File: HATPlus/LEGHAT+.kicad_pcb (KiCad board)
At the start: 4 copper layers, 65 x 56.5 mm, 28 parts, among them J1 Conn_02x20_Odd_Even, J2 Conn_01x02, J3 Conn_01x08, Q2 CSD18540Q5B, SW1 SW_Push, U4 LTC4373IDD-PBF

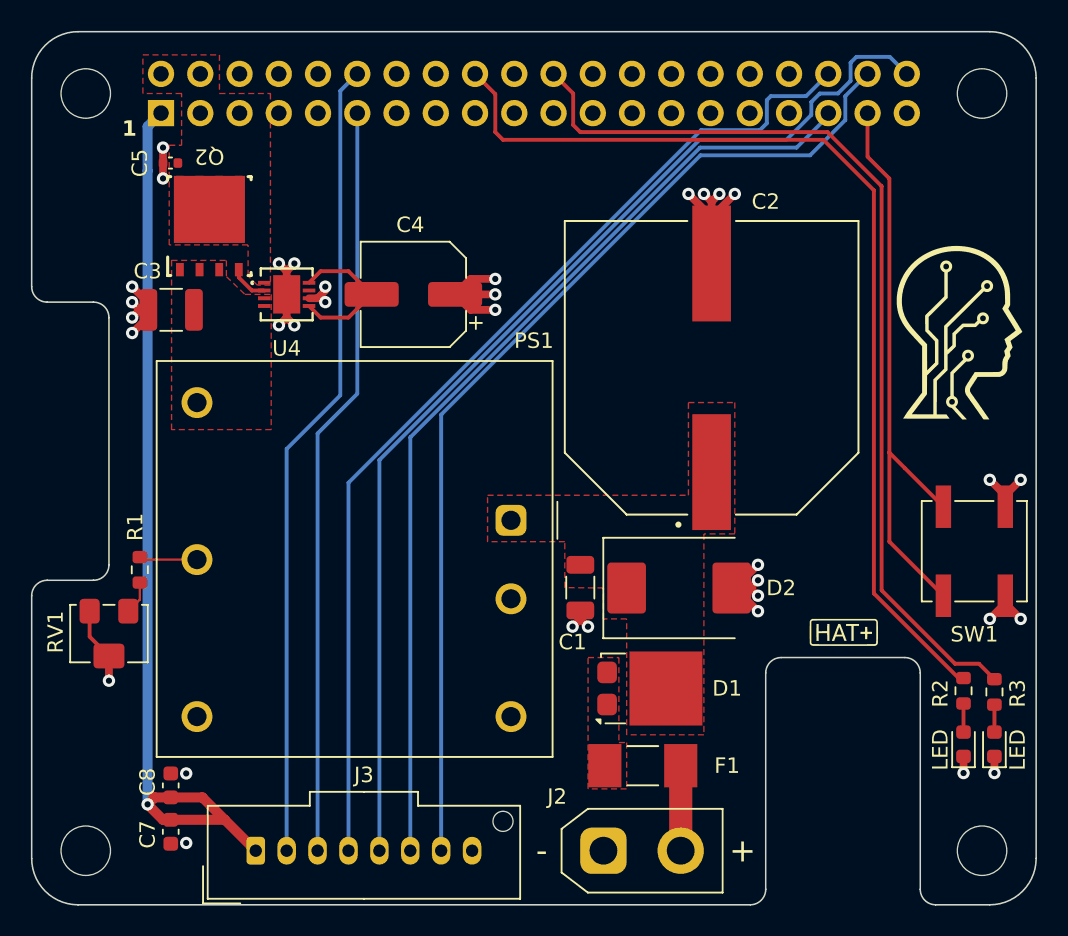
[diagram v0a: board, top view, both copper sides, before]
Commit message: First Draft
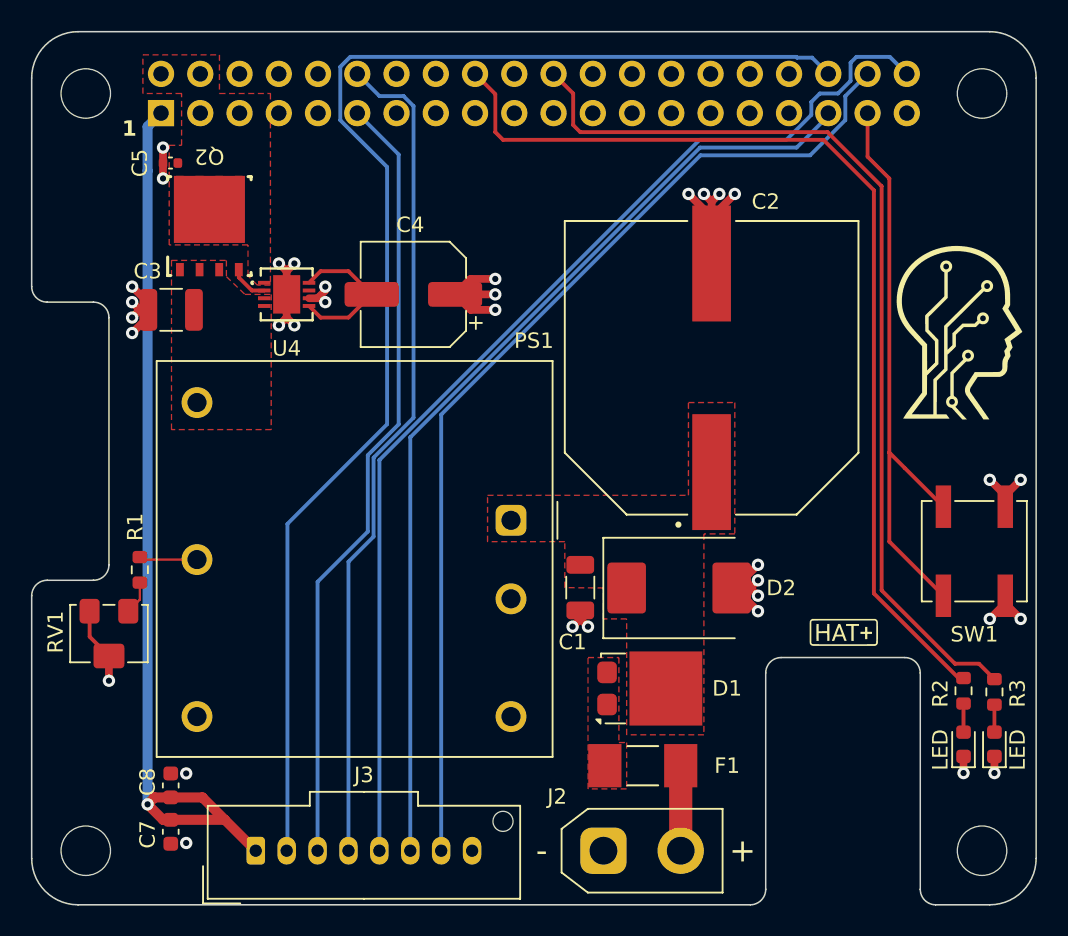
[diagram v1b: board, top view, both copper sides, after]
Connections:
- J1 pad 12: /SPI1_CSn2 -> /SPI1_CSn0
- J1 pad 36: /SPI1_CSn0 -> /SPI1_CSn2
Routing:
- net /SPI1_CSn2: track 52.2 -> 87.0 mm
- net /SPI1_CSn0: track 66.7 -> 54.4 mm
- net /SPI1_CSn1: track 48.8 -> 51.0 mm
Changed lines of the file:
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@@
 			(layers "*.Cu" "*.Mask")
 			(remove_unused_layers no)
-			(net "/SPI1_CSn2")
+			(net "/SPI1_CSn0")
 			(pinfunction "Pin_12_12")
 			(pintype "passive")
@@
 			(layers "*.Cu" "*.Mask")
 			(remove_unused_layers no)
-			(net "/SPI1_CSn0")
+			(net "/SPI1_CSn2")
 			(pinfunction "Pin_36_36")
 			(pintype "passive")
@@
 	)
 	(segment
+		(start 19.97 2.274365)
+		(end 19.97 5.725635)
+		(width 0.25)
+		(layer "B.Cu")
+		(net "/SPI1_CSn2")
+	)
+	(segment
+		(start 51.55 2.73)
+		(end 50.5 1.68)
+		(width 0.25)
+		(layer "B.Cu")
+		(net "/SPI1_CSn2")
+	)
+	(segment
+		(start 49.515635 1.68)
+		(end 49.465635 1.63)
+		(width 0.25)
+		(layer "B.Cu")
+		(net "/SPI1_CSn2")
+	)
+	(segment
+		(start 20.614365 1.63)
+		(end 19.97 2.274365)
+		(width 0.25)
+		(layer "B.Cu")
+		(net "/SPI1_CSn2")
+	)
+	(segment
+		(start 23 8.755635)
+		(end 23 25.4)
+		(width 0.25)
+		(layer "B.Cu")
+		(net "/SPI1_CSn2")
+	)
+	(segment
+		(start 19.97 5.725635)
+		(end 23 8.755635)
+		(width 0.25)
+		(layer "B.Cu")
+		(net "/SPI1_CSn2")
+	)
+	(segment
+		(start 16.55 52.95)
+		(end 16.5 53)
+		(width 0.15)
+		(layer "B.Cu")
+		(net "/SPI1_CSn2")
+	)
+	(segment
+		(start 16.55 31.85)
+		(end 16.55 52.95)
+		(width 0.25)
+		(layer "B.Cu")
+		(net "/SPI1_CSn2")
+	)
+	(segment
+		(start 23 25.4)
+		(end 16.55 31.85)
+		(width 0.25)
+		(layer "B.Cu")
+		(net "/SPI1_CSn2")
+	)
+	(segment
+		(start 50.5 1.68)
+		(end 49.515635 1.68)
+		(width 0.25)
+		(layer "B.Cu")
+		(net "/SPI1_CSn2")
+	)
+	(segment
+		(start 49.465635 1.63)
+		(end 20.614365 1.63)
+		(width 0.25)
+		(layer "B.Cu")
+		(net "/SPI1_CSn2")
+	)
+	(segment
+		(start 23.75 25.40901)
+		(end 21.75 27.40901)
+		(width 0.25)
+		(layer "B.Cu")
+		(net "/SPI1_CSn1")
+	)
+	(segment
+		(start 23.75 7.95)
+		(end 23.75 25.40901)
+		(width 0.25)
+		(layer "B.Cu")
+		(net "/SPI1_CSn1")
+	)
+	(segment
+		(start 18.5 35.6)
+		(end 18.5 53)
+		(width 0.25)
+		(layer "B.Cu")
+		(net "/SPI1_CSn1")
+	)
+	(segment
+		(start 21.07 5.27)
+		(end 23.75 7.95)
+		(width 0.25)
+		(layer "B.Cu")
+		(net "/SPI1_CSn1")
+	)
+	(segment
+		(start 21.75 27.40901)
+		(end 21.75 32.35)
+		(width 0.25)
+		(layer "B.Cu")
+		(net "/SPI1_CSn1")
+	)
+	(segment
+		(start 21.75 32.35)
+		(end 18.5 35.6)
+		(width 0.25)
+		(layer "B.Cu")
+		(net "/SPI1_CSn1")
+	)
+	(segment
+		(start 24.71 4.814365)
+		(end 24.71 24.97934)
+		(width 0.25)
+		(layer "B.Cu")
+		(net "/SPI1_CSn0")
+	)
+	(segment
+		(start 20.5 34.3)
+		(end 20.5 53)
+		(width 0.25)
+		(layer "B.Cu")
+		(net "/SPI1_CSn0")
+	)
+	(segment
+		(start 24.065635 4.17)
+		(end 24.71 4.814365)
+		(width 0.25)
+		(layer "B.Cu")
+		(net "/SPI1_CSn0")
+	)
+	(segment
 		(start 21.07 2.73)
-		(end 19.97 3.83)
-		(width 0.25)
-		(layer "B.Cu")
-		(net "/SPI1_CSn2")
-	)
-	(segment
-		(start 19.97 23.53)
-		(end 16.5 27)
-		(width 0.25)
-		(layer "B.Cu")
-		(net "/SPI1_CSn2")
-	)
-	(segment
-		(start 19.97 3.83)
-		(end 19.97 23.53)
-		(width 0.25)
-		(layer "B.Cu")
-		(net "/SPI1_CSn2")
-	)
-	(segment
-		(start 16.5 27)
-		(end 16.5 53)
-		(width 0.25)
-		(layer "B.Cu")
-		(net "/SPI1_CSn2")
-	)
-	(segment
-		(start 21.07 23.43)
-		(end 18.5 26)
-		(width 0.25)
-		(layer "B.Cu")
-		(net "/SPI1_CSn1")
-	)
-	(segment
-		(start 21.07 5.27)
-		(end 21.07 23.43)
-		(width 0.25)
-		(layer "B.Cu")
-		(net "/SPI1_CSn1")
-	)
-	(segment
-		(start 18.5 26)
-		(end 18.5 53)
-		(width 0.25)
-		(layer "B.Cu")
-		(net "/SPI1_CSn1")
-	)
-	(segment
-		(start 47.83 4.17)
-		(end 47.57 4.43)
+		(end 22.51 4.17)
 		(width 0.25)
 		(layer "B.Cu")
@@
 	)
 	(segment
-		(start 20.5 29.18934)
-		(end 20.5 53)
+		(start 22.51 4.17)
+		(end 24.065635 4.17)
 		(width 0.25)
 		(layer "B.Cu")
@@
 	)
 	(segment
-		(start 47.57 4.43)
-		(end 47.57 5.93)
+		(start 24.71 24.97934)
+		(end 22.125 27.56434)
 		(width 0.25)
 		(layer "B.Cu")
@@
 	)
 	(segment
-		(start 43.31934 6.37)
-		(end 20.5 29.18934)
+		(start 22.125 27.56434)
+		(end 22.125 32.675)
 		(width 0.25)
 		(layer "B.Cu")
@@
 	)
 	(segment
-		(start 51.55 2.73)
-		(end 50.11 4.17)
-		(width 0.25)
-		(layer "B.Cu")
-		(net "/SPI1_CSn0")
-	)
-	(segment
-		(start 47.57 5.93)
-		(end 47.13 6.37)
-		(width 0.25)
-		(layer "B.Cu")
-		(net "/SPI1_CSn0")
-	)
-	(segment
-		(start 50.11 4.17)
-		(end 47.83 4.17)
-		(width 0.25)
-		(layer "B.Cu")
-		(net "/SPI1_CSn0")
-	)
-	(segment
-		(start 47.13 6.37)
-		(end 43.31934 6.37)
-		(width 0.25)
-		(layer "B.Cu")
+		(start 22.125 32.675)
+		(end 20.5 34.3)
+		(width 0.25)
+		(layer "B.Cu")

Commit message: Draft 2
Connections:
- net /USB_Switch renamed /PWR_Switch
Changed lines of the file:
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@@
 			(size 2.75 1)
 			(layers "F.Cu" "F.Mask" "F.Paste")
-			(net "/USB_Switch")
+			(net "/PWR_Switch")
 			(pinfunction "1_1")
 			(pintype "passive")
@@
 			(size 2.75 1)
 			(layers "F.Cu" "F.Mask" "F.Paste")
-			(net "/USB_Switch")
+			(net "/PWR_Switch")
 			(pinfunction "1_1")
 			(pintype "passive")
@@
 			(layers "*.Cu" "*.Mask")
 			(remove_unused_layers no)
-			(net "/USB_Switch")
+			(net "/PWR_Switch")
 			(pinfunction "Pin_37_37")
 			(pintype "passive")
@@
 	)
 	(segment
-		(start 59 30.74)
-		(end 56.5 28.24)
-		(width 0.25)
-		(layer "F.Cu")
-		(net "/USB_Switch")
-	)
-	(segment
-		(start 54.09 8.09)
-		(end 54.09 5.27)
-		(width 0.25)
-		(layer "F.Cu")
-		(net "/USB_Switch")
-	)
-	(segment
-		(start 55.5 27.24)
-		(end 55.5 9.5)
-		(width 0.25)
-		(layer "F.Cu")
-		(net "/USB_Switch")
-	)
-	(segment
-		(start 55.5 33)
-		(end 55.5 27.24)
-		(width 0.25)
-		(layer "F.Cu")
-		(net "/USB_Switch")
-	)
-	(segment
-		(start 59 36.5)
-		(end 55.5 33)
-		(width 0.25)
-		(layer "F.Cu")
-		(net "/USB_Switch")
-	)
-	(segment
-		(start 55.5 9.5)
-		(end 54.09 8.09)
-		(width 0.25)
-		(layer "F.Cu")
-		(net "/USB_Switch")
-	)
-	(segment
-		(start 56.5 28.24)
-		(end 55.5 27.24)
-		(width 0.25)
-		(layer "F.Cu")
-		(net "/USB_Switch")
-	)
-	(segment
 		(start 10.6975 34.16)
 		(end 7.16 34.16)
@@
 		(net "/RED_LED")
 	)
+	(segment
+		(start 59 30.74)
+		(end 56.5 28.24)
+		(width 0.25)
+		(layer "F.Cu")
+		(net "/PWR_Switch")
+	)
+	(segment
+		(start 54.09 8.09)
+		(end 54.09 5.27)
+		(width 0.25)
+		(layer "F.Cu")
+		(net "/PWR_Switch")
+	)
+	(segment
+		(start 55.5 27.24)
+		(end 55.5 9.5)
+		(width 0.25)
+		(layer "F.Cu")
+		(net "/PWR_Switch")
+	)
+	(segment
+		(start 55.5 33)
+		(end 55.5 27.24)
+		(width 0.25)
+		(layer "F.Cu")
+		(net "/PWR_Switch")
+	)
+	(segment
+		(start 59 36.5)
+		(end 55.5 33)
+		(width 0.25)
+		(layer "F.Cu")
+		(net "/PWR_Switch")
+	)
+	(segment
+		(start 55.5 9.5)
+		(end 54.09 8.09)
+		(width 0.25)
+		(layer "F.Cu")
+		(net "/PWR_Switch")
+	)
+	(segment
+		(start 56.5 28.24)
+		(end 55.5 27.24)
+		(width 0.25)
+		(layer "F.Cu")
+		(net "/PWR_Switch")
+	)
 	(zone
